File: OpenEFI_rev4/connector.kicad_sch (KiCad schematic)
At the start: 56 parts, among them J6 1241434-1, Q10 PMN30XPX, Q20 PMN30XPX, Q5 SS8050, Q6 IRLZ44N, Q7 IRLZ44N, U14 MIC5205-3.3YM5, U16 TPS5430DDA, U17 L78M05ABDT-TR, U6 LT4363IMS

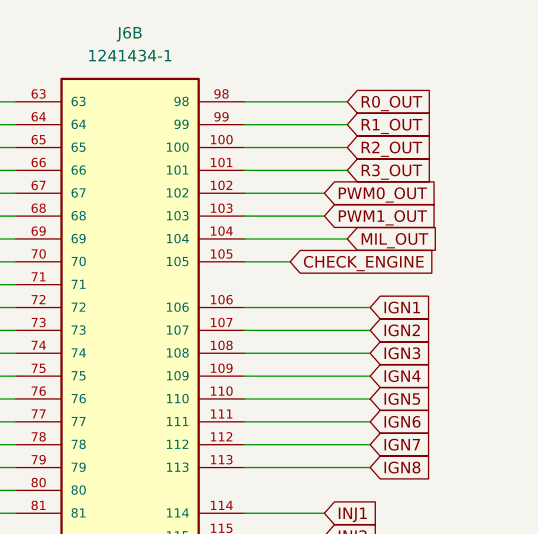
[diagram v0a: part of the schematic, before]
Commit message: WIP relay driver
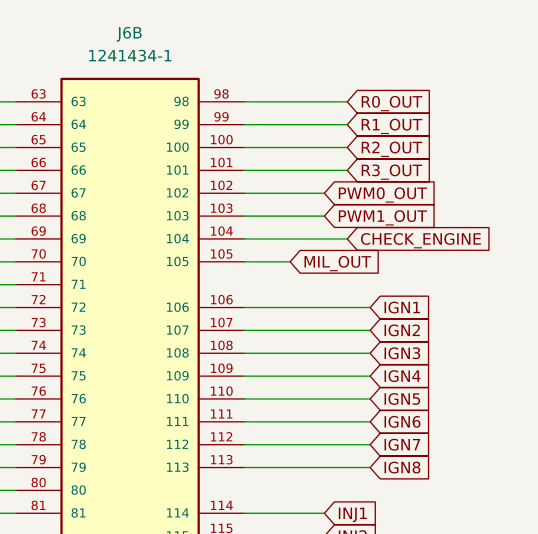
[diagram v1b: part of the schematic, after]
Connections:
- net CHECK_ENGINE: now also J6.104; no longer J6.105
- net MIL_OUT: now also J6.105; no longer J6.104
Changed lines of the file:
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@@
     )
   )
-  (global_label "MIL_OUT" (shape input) (at 267.97 43.18 0)
-    (effects (font (size 1.27 1.27)) (justify left))
-    (property "Intersheetrefs" "${INTERSHEET_REFS}" (at 272.8626 43.1006 0)
+  (global_label "MIL_OUT" (shape input) (at 261.62 45.72 0)
+    (effects (font (size 1.27 1.27)) (justify left))
+    (property "Intersheetrefs" "${INTERSHEET_REFS}" (at 266.5126 45.6406 0)
       (effects (font (size 1.27 1.27)) (justify left) hide)
     )
@@
     )
   )
-  (global_label "CHECK_ENGINE" (shape input) (at 261.62 45.72 0)
-    (effects (font (size 1.27 1.27)) (justify left))
-    (property "Intersheetrefs" "${INTERSHEET_REFS}" (at 266.3917 45.6406 0)
-      (effects (font (size 1.27 1.27)) (justify left) hide)
-    )
+  (global_label "CHECK_ENGINE" (shape input) (at 267.97 43.18 0)
+    (effects (font (size 1.27 1.27)) (justify left))
+    (property "Intersheetrefs" "${INTERSHEET_REFS}" (at 272.7417 43.1006 0)
+      (effects (font (size 1.27 1.27)) (justify left) hide)
+    )
